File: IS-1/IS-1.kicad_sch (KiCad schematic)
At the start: 0 parts

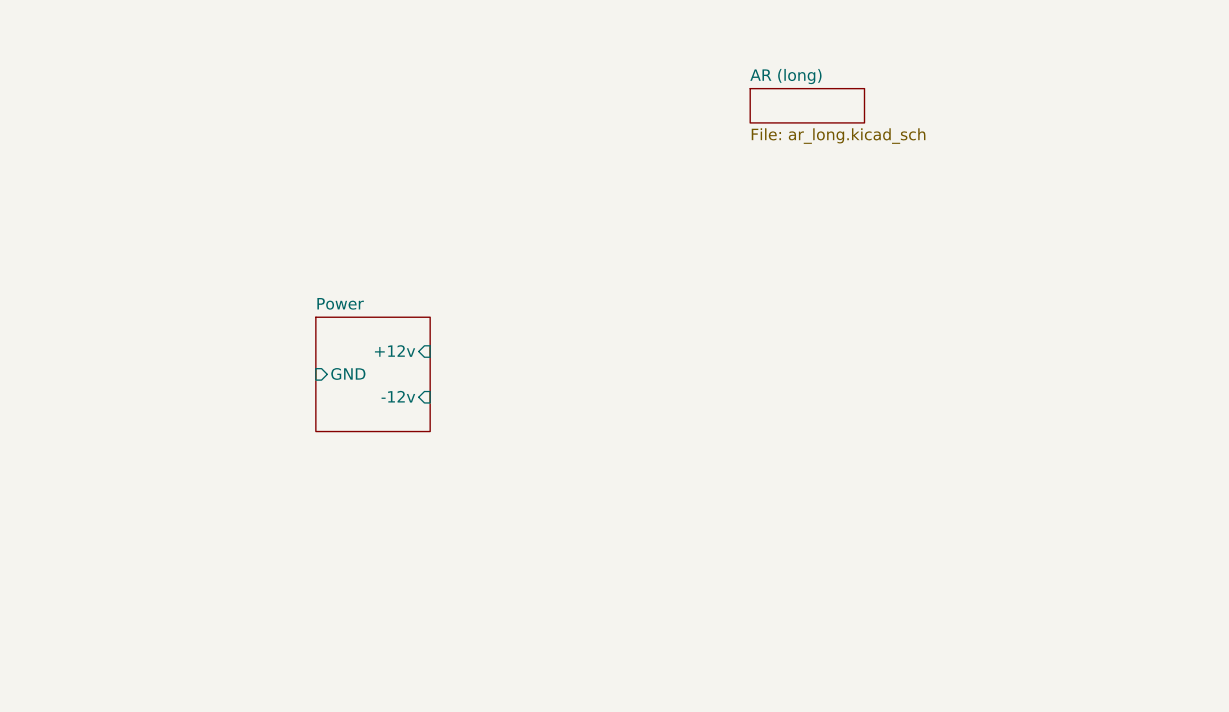
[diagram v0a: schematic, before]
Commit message: update
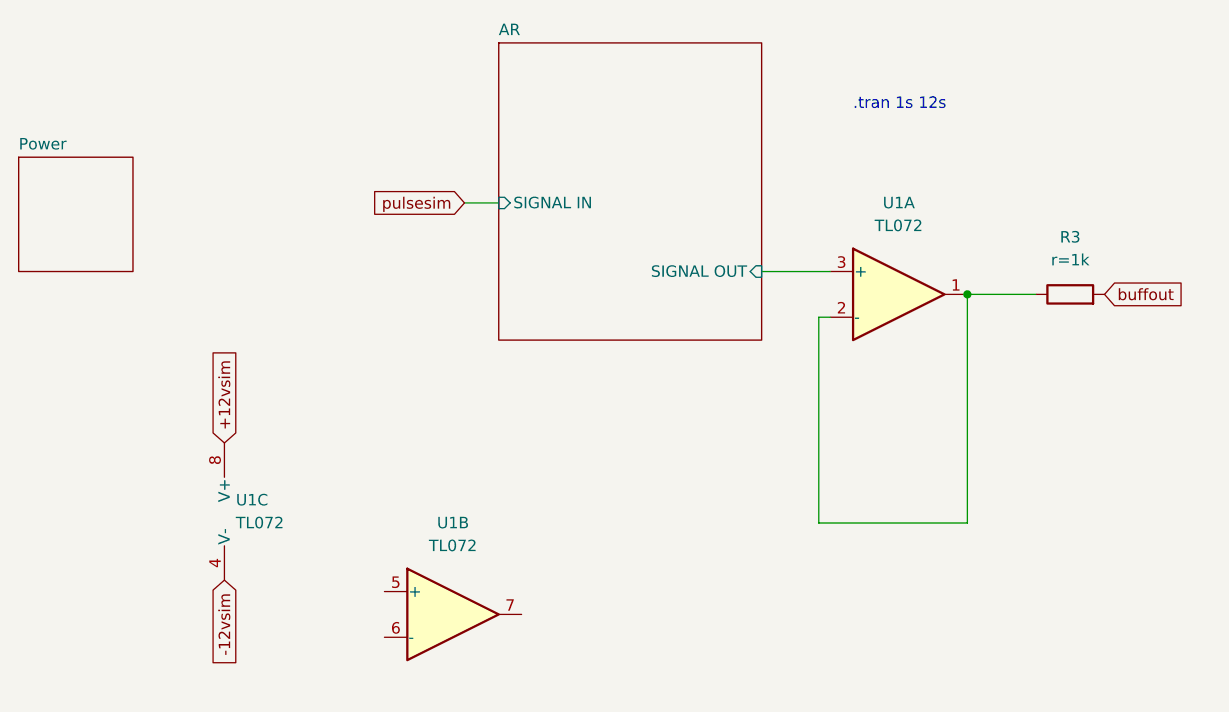
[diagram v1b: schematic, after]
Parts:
- added R3: ${SIM.PARAMS}, symbol Device:R
- added U1: TL072, symbol Amplifier_Operational:TL072
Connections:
- new net: R3.1, U1.1, U1.2 (-)
- new net +12vsim: U1.8 (V+)
- new net -12vsim: U1.4 (V-)
- new net AR/SIGNAL OUT: U1.3 (+)
- new net buffout: R3.2
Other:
- sheet AR (long) renamed AR
- sheet AR ports: added SIGNAL IN, SIGNAL OUT; removed none
- sheet Power ports: added none; removed +12v, -12v, GND
- note added: ".tran 1s 12s"
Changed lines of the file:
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@@
 (kicad_sch (version 20230121) (generator eeschema)
   (paper "A4")
-  (sheet (at 139.7 49.53) (size 12.7 3.81) (fields_autoplaced)
+  (junction (at 163.83 72.39) (diameter 0) (color 0 0 0 0)
+  )
+  (wire (pts (xy 163.83 72.39) (xy 163.83 97.79))
+    (stroke (width 0) (type default))
+  )
+  (wire (pts (xy 140.97 69.85) (xy 148.59 69.85))
+    (stroke (width 0) (type default))
+  )
+  (wire (pts (xy 147.32 74.93) (xy 148.59 74.93))
+    (stroke (width 0) (type default))
+  )
+  (wire (pts (xy 107.95 62.23) (xy 111.76 62.23))
+    (stroke (width 0) (type default))
+  )
+  (wire (pts (xy 163.83 72.39) (xy 171.45 72.39))
+    (stroke (width 0) (type default))
+  )
+  (wire (pts (xy 147.32 97.79) (xy 147.32 74.93))
+    (stroke (width 0) (type default))
+  )
+  (wire (pts (xy 163.83 97.79) (xy 147.32 97.79))
+    (stroke (width 0) (type default))
+  )
+  (text ".tran 1s 12s" (at 151.13 52.07 0)
+    (effects (font (size 1.27 1.27)) (justify left bottom))
+  )
+  (global_label "pulsesim" (shape input) (at 107.95 62.23 180) (fields_autoplaced)
+    (effects (font (size 1.27 1.27)) (justify right))
+    (property "Intersheetrefs" "${INTERSHEET_REFS}" (at 96.5587 62.23 0)
+      (effects (font (size 1.27 1.27)) (justify right) hide)
+    )
+  )
+  (global_label "+12vsim" (shape input) (at 81.28 88.9 90) (fields_autoplaced)
+    (effects (font (size 1.27 1.27)) (justify left))
+    (property "Intersheetrefs" "${INTERSHEET_REFS}" (at 81.28 77.6296 90)
+      (effects (font (size 1.27 1.27)) (justify left) hide)
+    )
+  )
+  (global_label "buffout" (shape input) (at 179.07 72.39 0) (fields_autoplaced)
+    (effects (font (size 1.27 1.27)) (justify left))
+    (property "Intersheetrefs" "${INTERSHEET_REFS}" (at 188.8283 72.39 0)
+      (effects (font (size 1.27 1.27)) (justify left) hide)
+    )
+  )
+  (global_label "-12vsim" (shape input) (at 81.28 104.14 270) (fields_autoplaced)
+    (effects (font (size 1.27 1.27)) (justify right))
+    (property "Intersheetrefs" "${INTERSHEET_REFS}" (at 81.28 115.4104 90)
+      (effects (font (size 1.27 1.27)) (justify right) hide)
+    )
+  )
+  (symbol (lib_id "Amplifier_Operational:TL072") (at 156.21 72.39 0) (unit 1)
+    (in_bom yes) (on_board yes) (dnp no) (fields_autoplaced)
+    (property "Reference" "U1" (at 156.21 62.23 0)
+      (effects (font (size 1.27 1.27)))
+    )
+    (property "Value" "TL072" (at 156.21 64.77 0)
+      (effects (font (size 1.27 1.27)))
+    )
+    (property "Footprint" "" (at 156.21 72.39 0)
+      (effects (font (size 1.27 1.27)) hide)
+    )
+    (property "Datasheet" "http://www.ti.com/lit/ds/symlink/tl071.pdf" (at 156.21 72.39 0)
+      (effects (font (size 1.27 1.27)) hide)
+    )
+    (property "Sim.Library" "/Users/chriscaragianis/projects/modules/spice_models/TL071_SN.lib" (at 156.21 72.39 0)
+      (effects (font (size 1.27 1.27)) hide)
+    )
+    (property "Sim.Name" "TL071_SN" (at 156.21 72.39 0)
+      (effects (font (size 1.27 1.27)) hide)
+    )
+    (property "Sim.Device" "SUBCKT" (at 156.21 72.39 0)
+      (effects (font (size 1.27 1.27)) hide)
+    )
+    (property "Sim.Pins" "1=5 2=2 3=1 4=4 8=3" (at 156.21 72.39 0)
+      (effects (font (size 1.27 1.27)) hide)
+    )
+    (pin "1")
+    (pin "2")
+    (pin "3")
+    (pin "5")
+    (pin "6")
+    (pin "7")
+    (pin "4")
+    (pin "8")
+    (instances
+      (project "IS-1"
+        (path "/733056ea-fa8c-44fe-a8d2-069ece4bafb9"
+          (reference "U1") (unit 1)
+        )
+      )
+    )
+  )
+  (symbol (lib_id "Amplifier_Operational:TL072") (at 83.82 96.52 0) (unit 3)
+    (in_bom yes) (on_board yes) (dnp no) (fields_autoplaced)
+    (property "Reference" "U1" (at 82.55 95.25 0)
+      (effects (font (size 1.27 1.27)) (justify left))
+    )
+    (property "Value" "TL072" (at 82.55 97.79 0)
+      (effects (font (size 1.27 1.27)) (justify left))
+    )
+    (property "Footprint" "" (at 83.82 96.52 0)
+      (effects (font (size 1.27 1.27)) hide)
+    )
+    (property "Datasheet" "http://www.ti.com/lit/ds/symlink/tl071.pdf" (at 83.82 96.52 0)
+      (effects (font (size 1.27 1.27)) hide)
+    )
+    (property "Sim.Library" "/Users/chriscaragianis/projects/modules/spice_models/TL071_SN.lib" (at 83.82 96.52 0)
+      (effects (font (size 1.27 1.27)) hide)
+    )
+    (property "Sim.Name" "TL071_SN" (at 83.82 96.52 0)
+      (effects (font (size 1.27 1.27)) hide)
+    )
+    (property "Sim.Device" "SUBCKT" (at 83.82 96.52 0)
+      (effects (font (size 1.27 1.27)) hide)
+    )
+    (property "Sim.Pins" "1=5 2=2 3=1 4=4 8=3" (at 83.82 96.52 0)
+      (effects (font (size 1.27 1.27)) hide)
+    )
+    (pin "1")
+    (pin "2")
+    (pin "3")
+    (pin "5")
+    (pin "6")
+    (pin "7")
+    (pin "4")
+    (pin "8")
+    (instances
+      (project "IS-1"
+        (path "/733056ea-fa8c-44fe-a8d2-069ece4bafb9"
+          (reference "U1") (unit 3)
+        )
+      )
+    )
+  )
+  (symbol (lib_id "Amplifier_Operational:TL072") (at 106.68 107.95 0) (unit 2)
+    (in_bom yes) (on_board yes) (dnp no) (fields_autoplaced)
+    (property "Reference" "U1" (at 106.68 97.79 0)
+      (effects (font (size 1.27 1.27)))
+    )
+    (property "Value" "TL072" (at 106.68 100.33 0)
+      (effects (font (size 1.27 1.27)))
+    )
+    (property "Footprint" "" (at 106.68 107.95 0)
+      (effects (font (size 1.27 1.27)) hide)
+    )
+    (property "Datasheet" "http://www.ti.com/lit/ds/symlink/tl071.pdf" (at 106.68 107.95 0)
+      (effects (font (size 1.27 1.27)) hide)
+    )
+    (property "Sim.Library" "/Users/chriscaragianis/projects/modules/spice_models/TL071_SN.lib" (at 106.68 107.95 0)
+      (effects (font (size 1.27 1.27)) hide)
+    )
+    (property "Sim.Name" "TL071_SN" (at 106.68 107.95 0)
+      (effects (font (size 1.27 1.27)) hide)
+    )
+    (property "Sim.Device" "SUBCKT" (at 106.68 107.95 0)
+      (effects (font (size 1.27 1.27)) hide)
+    )
+    (property "Sim.Pins" "1=5 2=2 3=1 4=4 8=3" (at 106.68 107.95 0)
+      (effects (font (size 1.27 1.27)) hide)
+    )
+    (pin "1")
+    (pin "2")
+    (pin "3")
+    (pin "5")
+    (pin "6")
+    (pin "7")
+    (pin "4")
+    (pin "8")
+    (instances
+      (project "IS-1"
+        (path "/733056ea-fa8c-44fe-a8d2-069ece4bafb9"
+          (reference "U1") (unit 2)
+        )
+      )
+    )
+  )
+  (symbol (lib_id "Device:R") (at 175.26 72.39 90) (unit 1)
+    (in_bom yes) (on_board yes) (dnp no) (fields_autoplaced)
+    (property "Reference" "R3" (at 175.26 66.04 90)
+      (effects (font (size 1.27 1.27)))
+    )
+    (property "Value" "${SIM.PARAMS}" (at 175.26 68.58 90)
+      (effects (font (size 1.27 1.27)))
+    )
+    (property "Footprint" "" (at 175.26 74.168 90)
+      (effects (font (size 1.27 1.27)) hide)
+    )
+    (property "Datasheet" "~" (at 175.26 72.39 0)
+      (effects (font (size 1.27 1.27)) hide)
+    )
+    (property "Sim.Device" "R" (at 175.26 72.39 0)
+      (effects (font (size 1.27 1.27)) hide)
+    )
+    (property "Sim.Type" "=" (at 175.26 72.39 0)
+      (effects (font (size 1.27 1.27)) hide)
+    )
+    (property "Sim.Params" "r=1k" (at 175.26 72.39 0)
+      (effects (font (size 1.27 1.27)) hide)
+    )
+    (property "Sim.Pins" "1=+ 2=-" (at 175.26 72.39 0)
+      (effects (font (size 1.27 1.27)) hide)
+    )
+    (pin "1")
+    (pin "2")
+    (instances
+      (project "IS-1"
+        (path "/733056ea-fa8c-44fe-a8d2-069ece4bafb9"
+          (reference "R3") (unit 1)
+        )
+      )
+    )
+  )
+  (sheet (at 111.76 44.45) (size 29.21 33.02) (fields_autoplaced)
     (stroke (width 0.1524) (type solid))
     (fill (color 0 0 0 0.0000))
-    (property "Sheetname" "AR (long)" (at 139.7 48.8184 0)
+    (property "Sheetname" "AR" (at 111.76 43.7384 0)
       (effects (font (size 1.27 1.27)) (justify left bottom))
     )
-    (property "Sheetfile" "ar_long.kicad_sch" (at 139.7 53.9246 0)
-      (effects (font (size 1.27 1.27)) (justify left top))
+    (property "Sheetfile" "ar_long.kicad_sch" (at 111.76 78.0546 0)
+      (effects (font (size 1.27 1.27)) (justify left top) hide)
+    )
+    (pin "SIGNAL IN" input (at 111.76 62.23 180)
+      (effects (font (size 1.27 1.27)) (justify left))
+    )
+    (pin "SIGNAL OUT" input (at 140.97 69.85 0)
+      (effects (font (size 1.27 1.27)) (justify right))
     )
     (instances
@@
     )
   )
-  (sheet (at 91.44 74.93) (size 12.7 12.7) (fields_autoplaced)
+  (sheet (at 58.42 57.15) (size 12.7 12.7) (fields_autoplaced)
     (stroke (width 0.1524) (type solid))
     (fill (color 0 0 0 0.0000))
-    (property "Sheetname" "Power" (at 91.44 74.2184 0)
+    (property "Sheetname" "Power" (at 58.42 56.4384 0)
       (effects (font (size 1.27 1.27)) (justify left bottom))
     )
-    (property "Sheetfile" "../subschema/10_pin_power/10_pin_power.kicad_sch" (at 91.44 88.2146 0)
+    (property "Sheetfile" "../subschema/10_pin_power/10_pin_power.kicad_sch" (at 58.42 70.4346 0)
       (effects (font (size 1.27 1.27)) (justify left top) hide)
     )
-    (pin "-12v" input (at 104.14 83.82 0)
-      (effects (font (size 1.27 1.27)) (justify right))
-    )
-    (pin "+12v" input (at 104.14 78.74 0)
-      (effects (font (size 1.27 1.27)) (justify right))
-    )
-    (pin "GND" input (at 91.44 81.28 180)
-      (effects (font (size 1.27 1.27)) (justify left))
-    )
-    (instances
+    (instances
